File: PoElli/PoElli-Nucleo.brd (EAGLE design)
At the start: 57.5 x 70 mm, 110 parts, among them J3 M022.54MM, J4 M022.54MM, Q3 FDMC2674HANDSOLDERING, Q4 FDMC2674HANDSOLDERING, T1 Coilcraft 230NL, T2 FLYBACK-3_OUTPUTS_749119350, U4 LT3748, U5 TPS2378, U6 ENC424J600, X1 POE-TP-SHIELDED-LEDSTE1888250, Y1 25 MHz

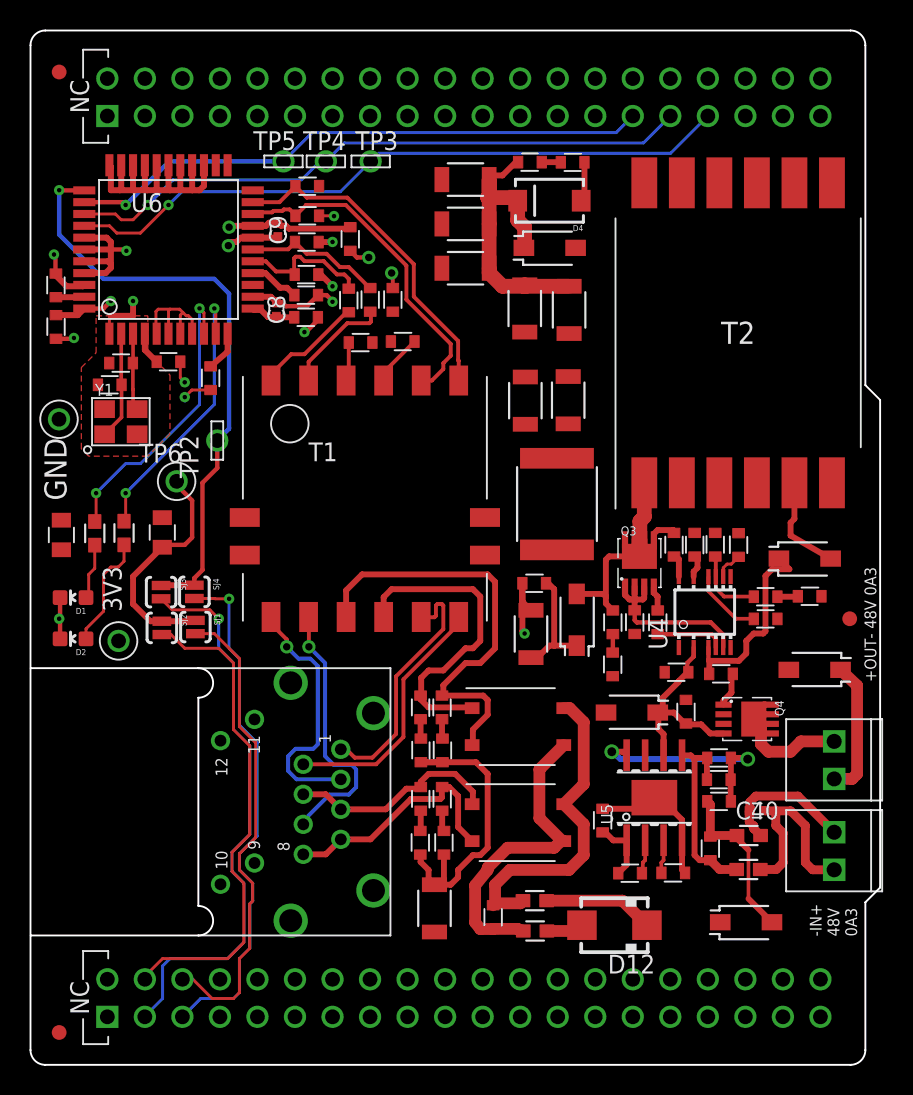
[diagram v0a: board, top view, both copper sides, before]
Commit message: component placement, planes final.
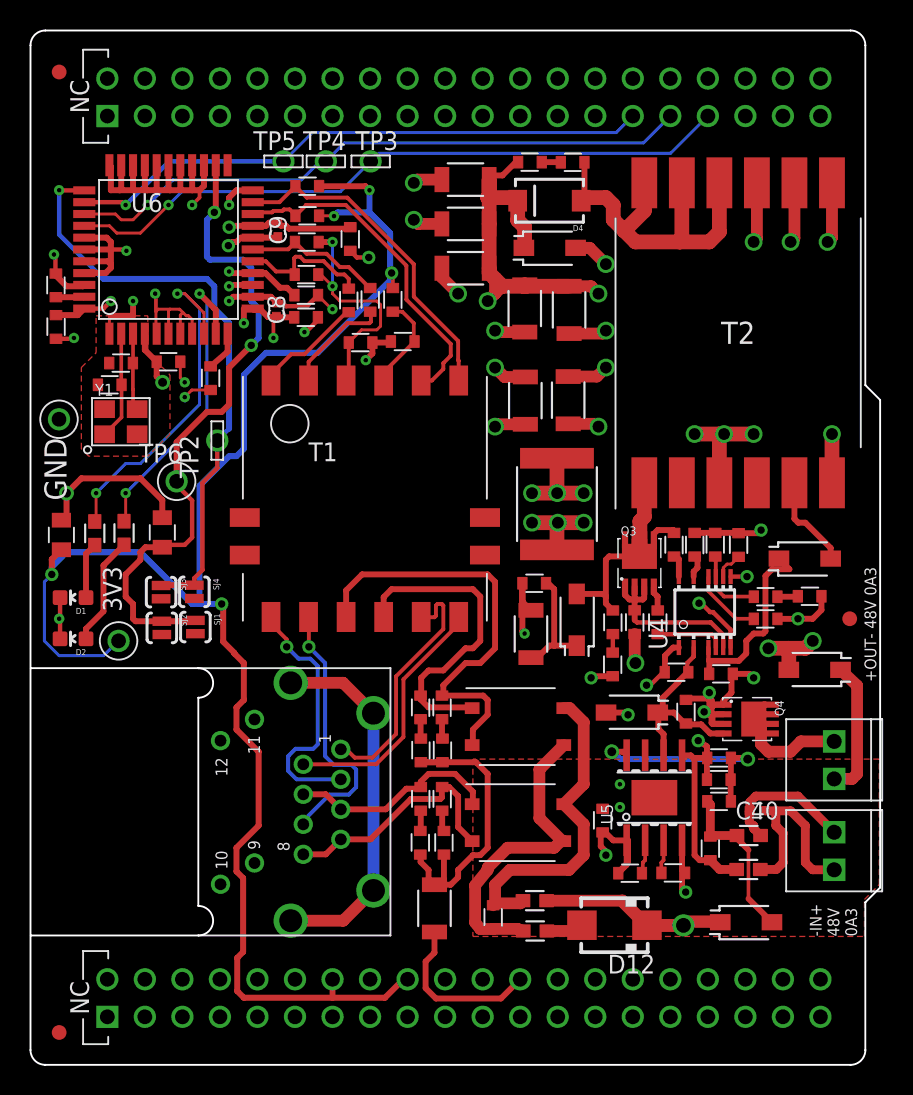
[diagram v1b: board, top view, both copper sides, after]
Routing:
- net +3V3: track 2.41 -> 113.2 mm, vias 2 -> 5
- net GNDA: track 76.4 -> 129.4 mm, vias 10 -> 27
- net RTN: track 15.4 -> 60.8 mm, vias 0 -> 17
- net N$11: track 38.2 -> 0.00 mm, vias 1 -> 0
- net VDD: track 17.4 -> 54.5 mm, vias 1 -> 12
- net N$12: track 35.6 -> 0.00 mm, vias 1 -> 0
- net N$13: track 33.7 -> 0.00 mm
- net N$14: track 32.5 -> 0.00 mm
- net ETH_INT: track 16.0 -> 44.9 mm, vias 0 -> 2
- net SGND: track 0.00 -> 24.9 mm
- net TRAFO_OUT: track 2.69 -> 25.4 mm
- net ENC-3V3: track 18.7 -> 40.0 mm, vias 3 -> 8
- net TPINCT: track 5.12 -> 16.1 mm
- net VIN: track 21.4 -> 32.0 mm, vias 0 -> 2
- net VSS: track 12.5 -> 7.65 mm, vias 0 -> 3
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- added copper zone on layer 2, net GNDA
- added copper zone on layer 2, net RTN
- added copper zone on layer 15, net VDD
- added copper zone on layer 15, net VIN
- added copper zone on layer 1, net VSS
- added copper zone on layer 2, net VSS
